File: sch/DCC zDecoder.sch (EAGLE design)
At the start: 25 parts, among them IC1 TSR 1-2450, IC2 ULN2803, IC3 ULN2803, J1 MPE 087-1-003, X1 DG240 2,54-8, X10 PSS 254/3G, X11 PSS 254/3G, X12 PSS 254/3G, X2 DG240 2,54-8, X3 DG240 2,54-8, X4 DG240 2,54-8, X5 DG240 2,54-2, X6 DG240 2,54-2, X7 PSS 254/3G, X8 PSS 254/3G, X9 PSS 254/3G

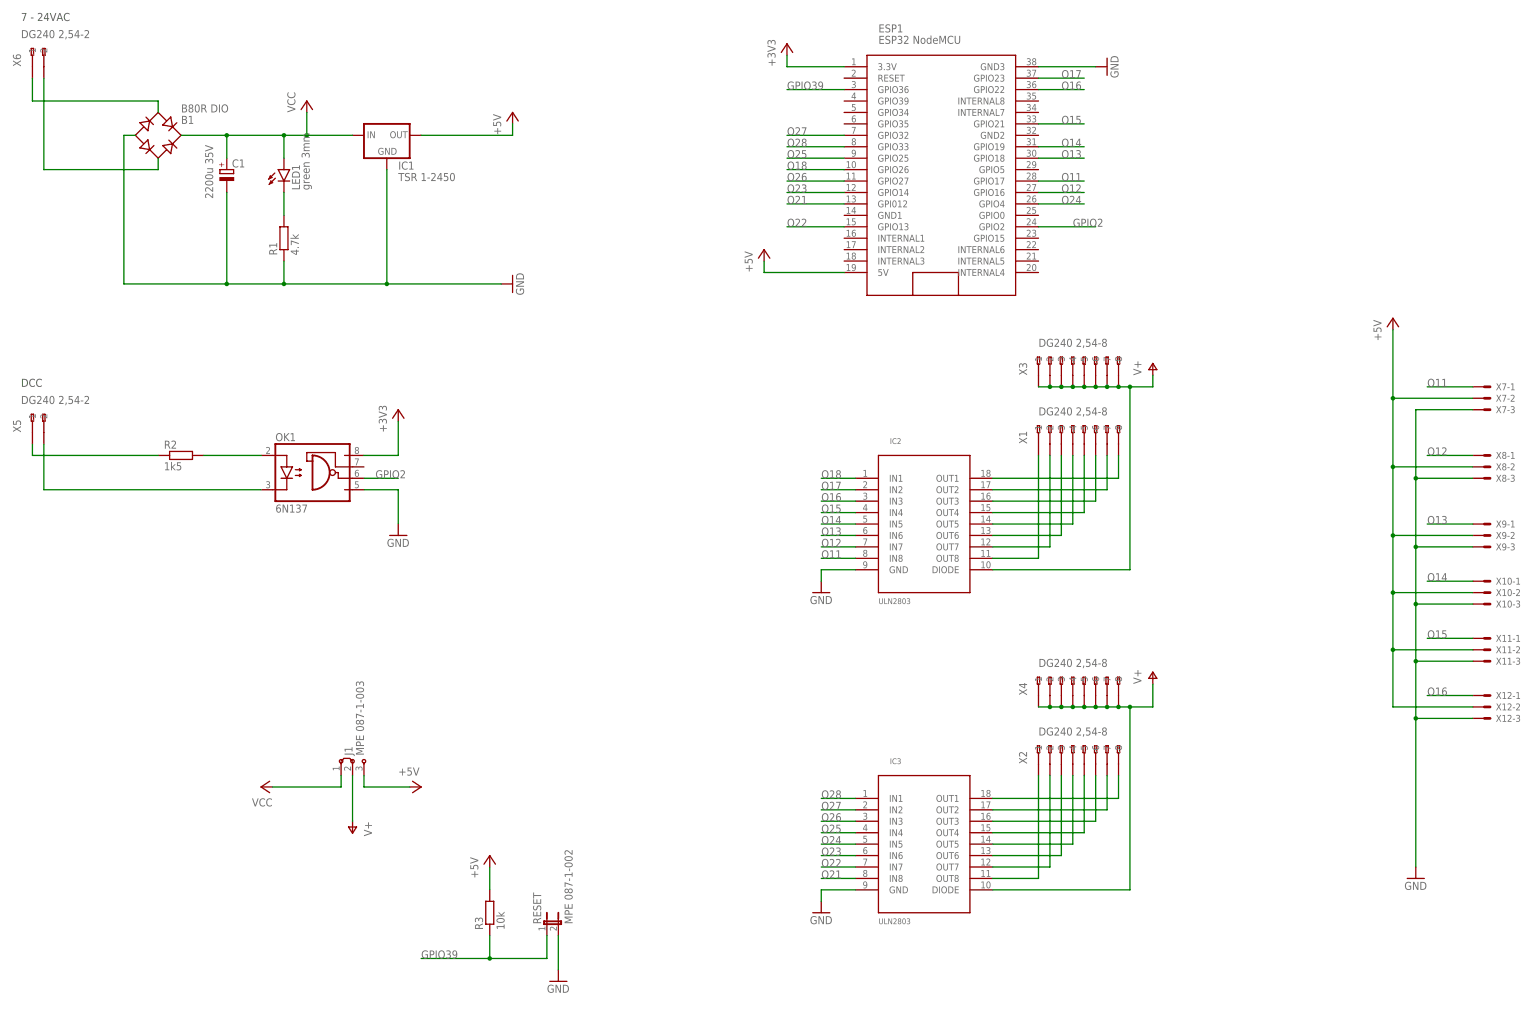
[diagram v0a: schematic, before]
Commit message: backup
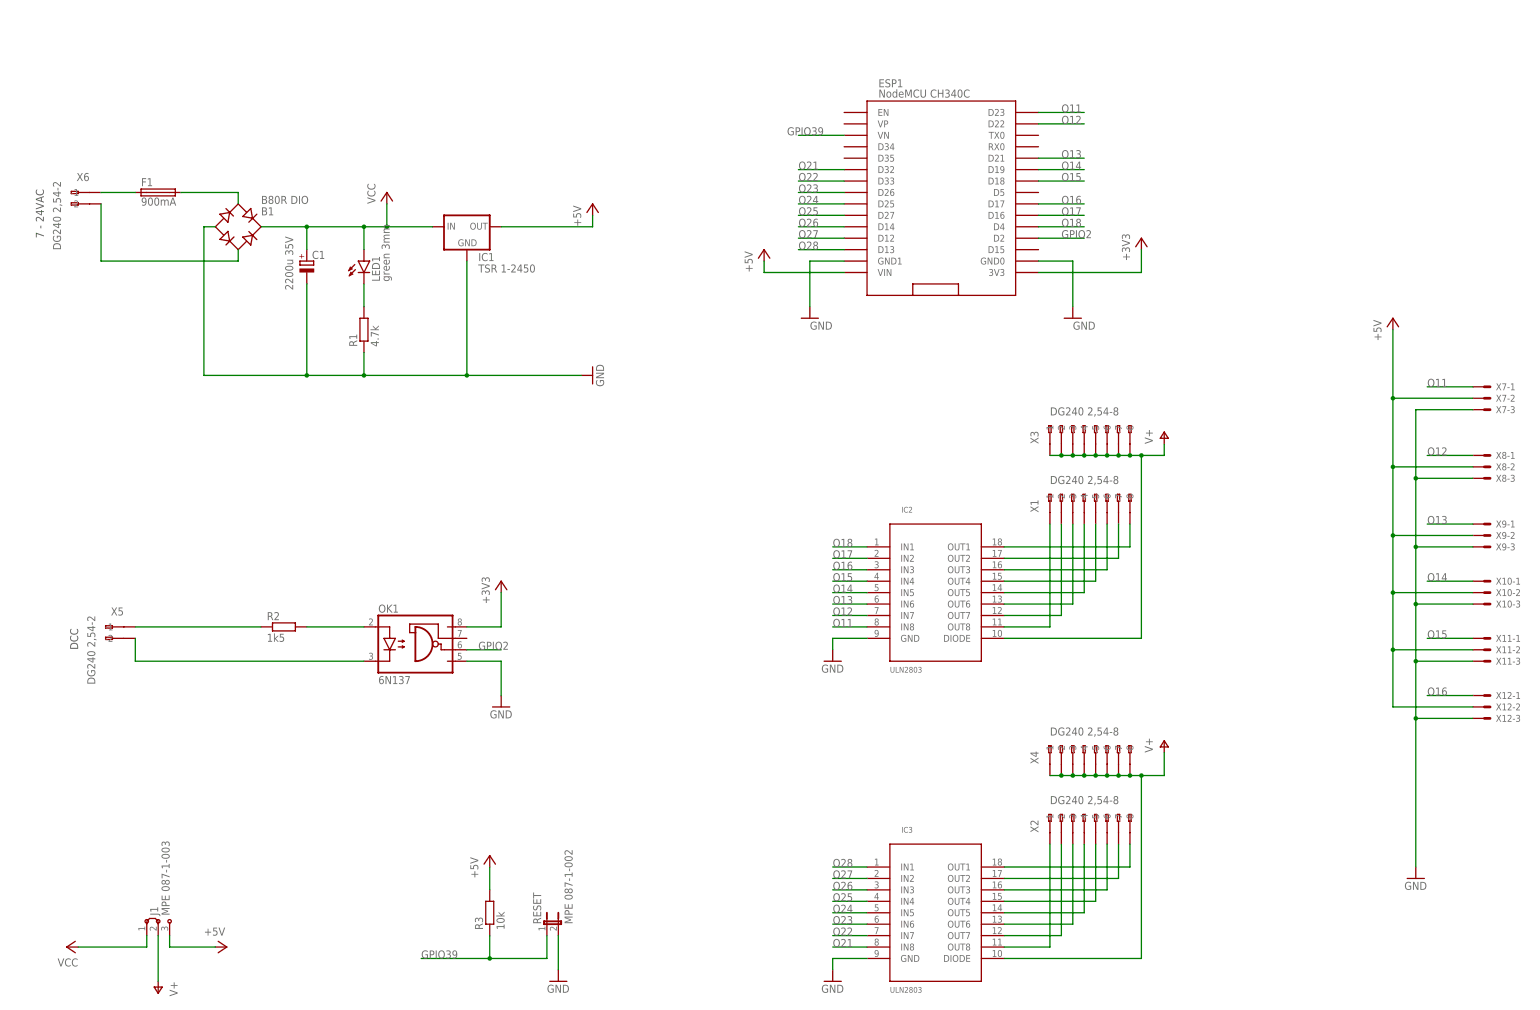
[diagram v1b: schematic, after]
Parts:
- added F1: 900mA, fuse:TE5
- ESP1: value ESP32 NodeMCU -> NodeMCU CH340C; device _esp32:ESP32-NODEMCU -> _esp32:ESP32-NODEMCU-CH340C
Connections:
- new net N$15: F1.1, X6.-1
- net +3V3: now also ESP1.3V3; no longer ESP1.3.3V
- net +5V: now also ESP1.VIN; no longer ESP1.5V
- net GND: now also ESP1.GND0, ESP1.GND1; no longer ESP1.GND3
- net GPIO2: now also ESP1.D2; no longer ESP1.GPIO2
- net GPIO39: now also ESP1.VN; no longer ESP1.GPIO36
- net N$5: now also F1.2; no longer X6.-1
- net O11: now also ESP1.D23; no longer ESP1.GPIO17
- net O12: now also ESP1.D22; no longer ESP1.GPIO16
- net O13: now also ESP1.D21; no longer ESP1.GPIO18
- net O14: now also ESP1.D19; no longer ESP1.GPIO19
- net O15: now also ESP1.D18; no longer ESP1.GPIO21
- net O16: now also ESP1.D17; no longer ESP1.GPIO22
- net O17: now also ESP1.D16; no longer ESP1.GPIO23
- net O18: now also ESP1.D4; no longer ESP1.GPIO26
- net O21: now also ESP1.D32; no longer ESP1.GPI012
- net O22: now also ESP1.D33; no longer ESP1.GPIO13
- net O23: now also ESP1.D26; no longer ESP1.GPIO14
- net O24: now also ESP1.D25; no longer ESP1.GPIO4
- net O25: now also ESP1.D27; no longer ESP1.GPIO25
- net O26: now also ESP1.D14; no longer ESP1.GPIO27
- net O27: now also ESP1.D12; no longer ESP1.GPIO32
- net O28: now also ESP1.D13; no longer ESP1.GPIO33
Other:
- moved on the sheet: B1, C1, IC1, IC2, IC3, J1, LED1, OK1, R1, R2, X1, X2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
